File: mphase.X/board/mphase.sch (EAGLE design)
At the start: 39 parts, among them IC1 MAX232, IC2 PIC18F4455_40, X1 332-10, X2 332-10

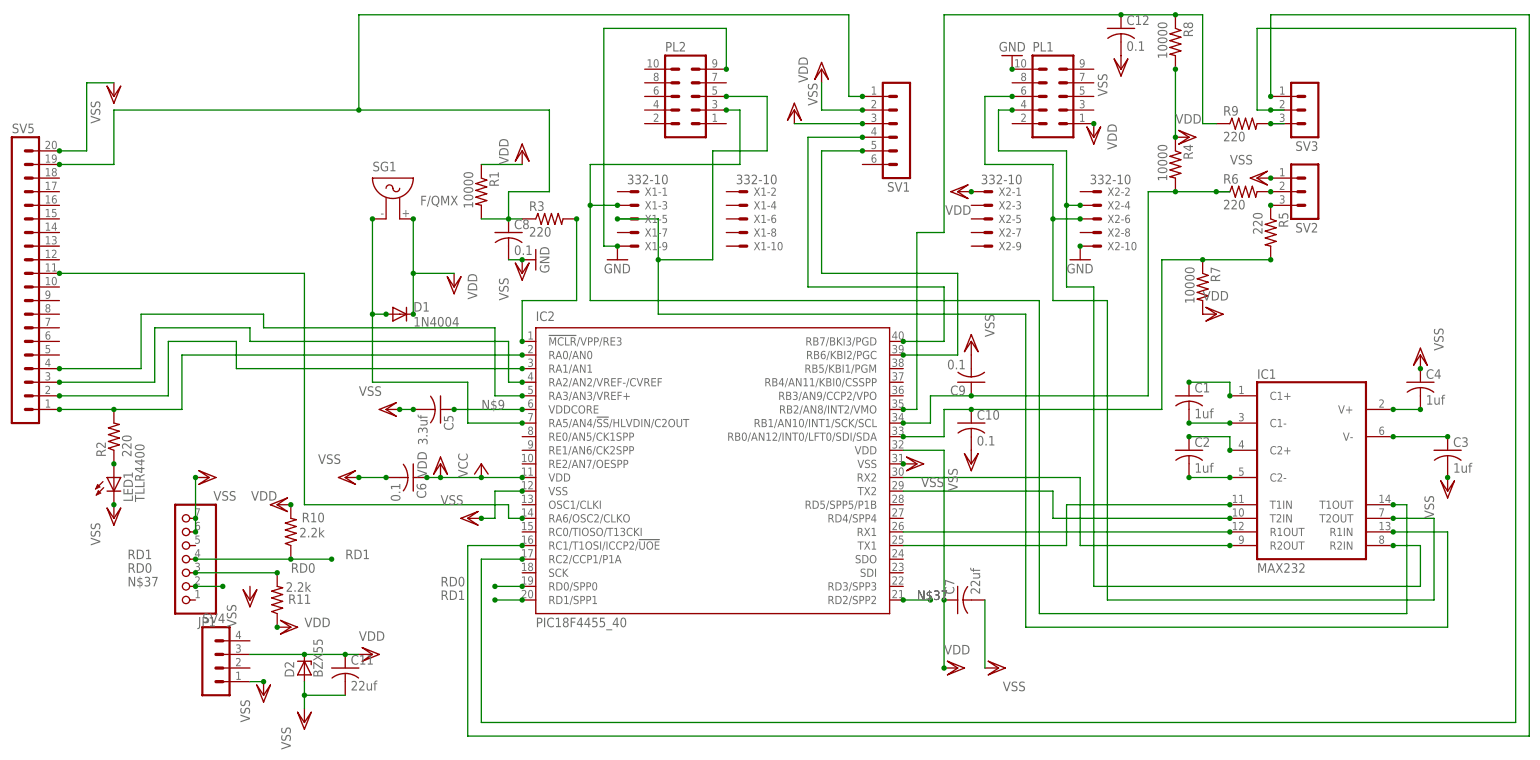
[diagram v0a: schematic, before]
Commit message: up
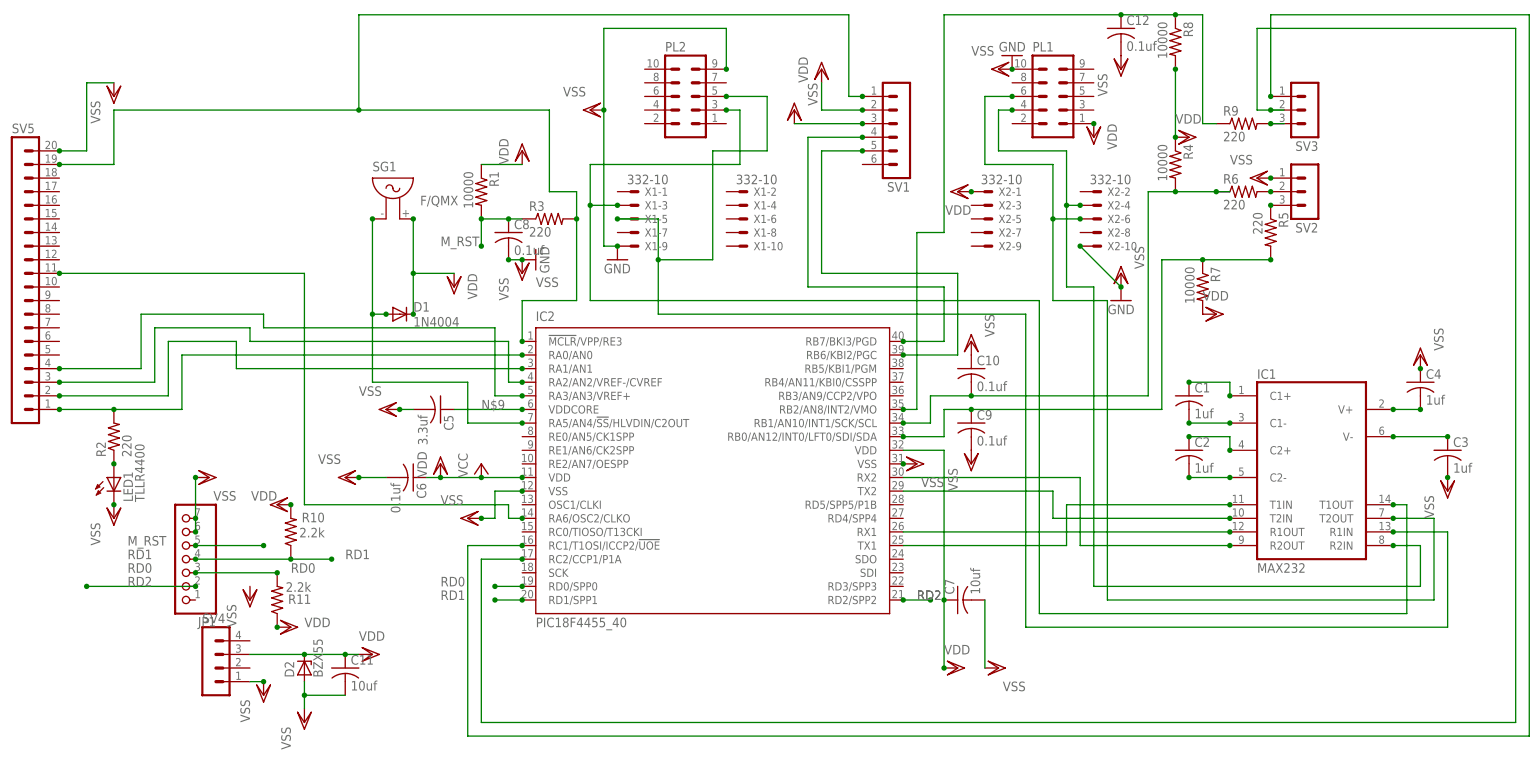
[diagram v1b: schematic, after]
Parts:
- C10, C12, C8, C9: value 0.1 -> 0.1uf; device resistor:C-US025-024X044 -> rcl:C-USC1206
- C11, C7: value 22uf -> 10uf; device resistor:C-US025-025X050 -> rcl:C-USC1206
- C5: device resistor:C-US025-025X050 -> rcl:C-USC1206
- C6: value 0.1 -> 0.1uf; device resistor:C-US025-025X050 -> rcl:C-USC1206
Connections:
- net N$37 renamed RD2
- removed net GND: C8.2, PL1.10, PL2.9, X1-9.S, X2-10.S
- removed net N$14: IC2.!MCLR!/VPP/RE3, R3.2
- new net M_RST: C8.1, JP1.5, R1.2, R3.1
- net N$21: now also C10.2; no longer C9.1
- net N$22: now also C9.1; no longer C10.1
- net N$8: now also IC2.!MCLR!/VPP/RE3, R3.2; no longer C8.1, R1.2, R3.1
- net VSS: now also C10.1, C8.2, PL1.10, PL2.9, X1-9.S, X2-10.S; no longer C10.2
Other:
- moved on the sheet: C10, C9
